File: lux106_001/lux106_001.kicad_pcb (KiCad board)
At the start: 2 copper layers, 19 parts, among them U1 40106, U2 LM324

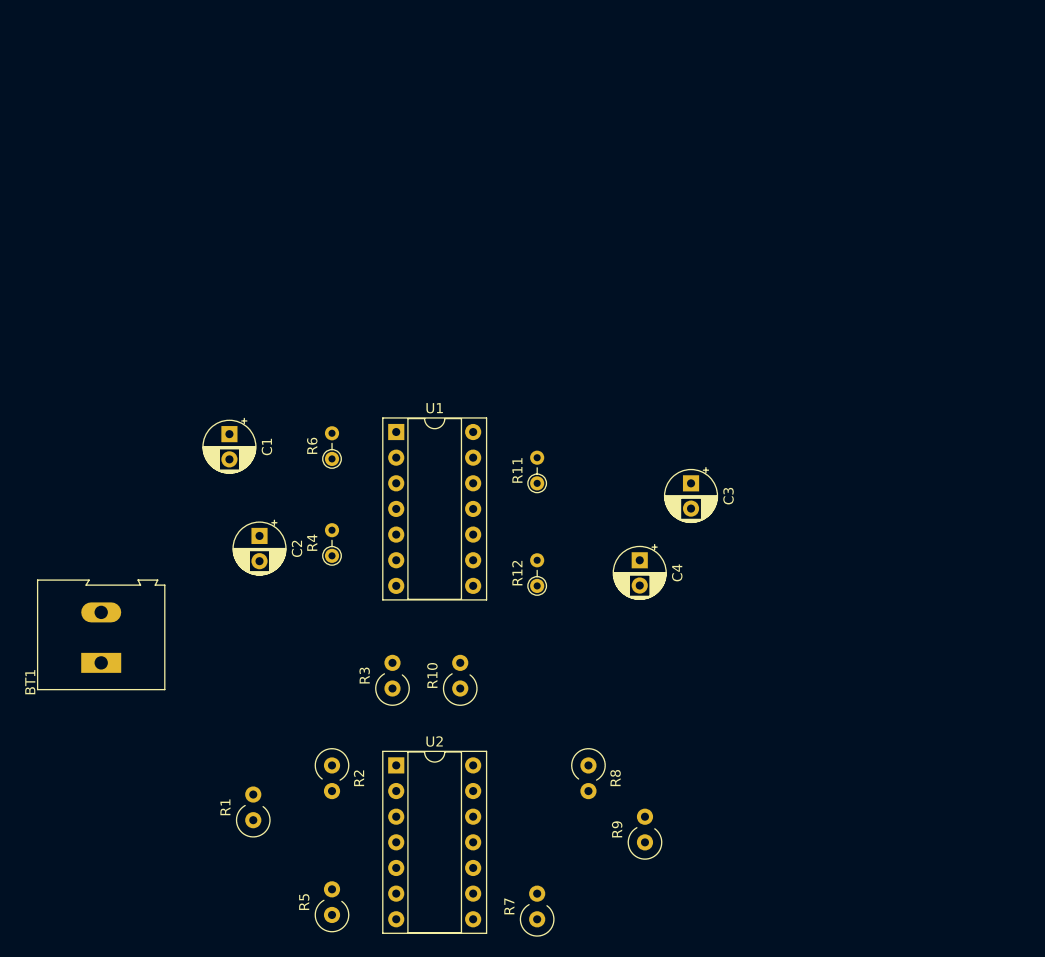
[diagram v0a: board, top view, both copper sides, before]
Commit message: update
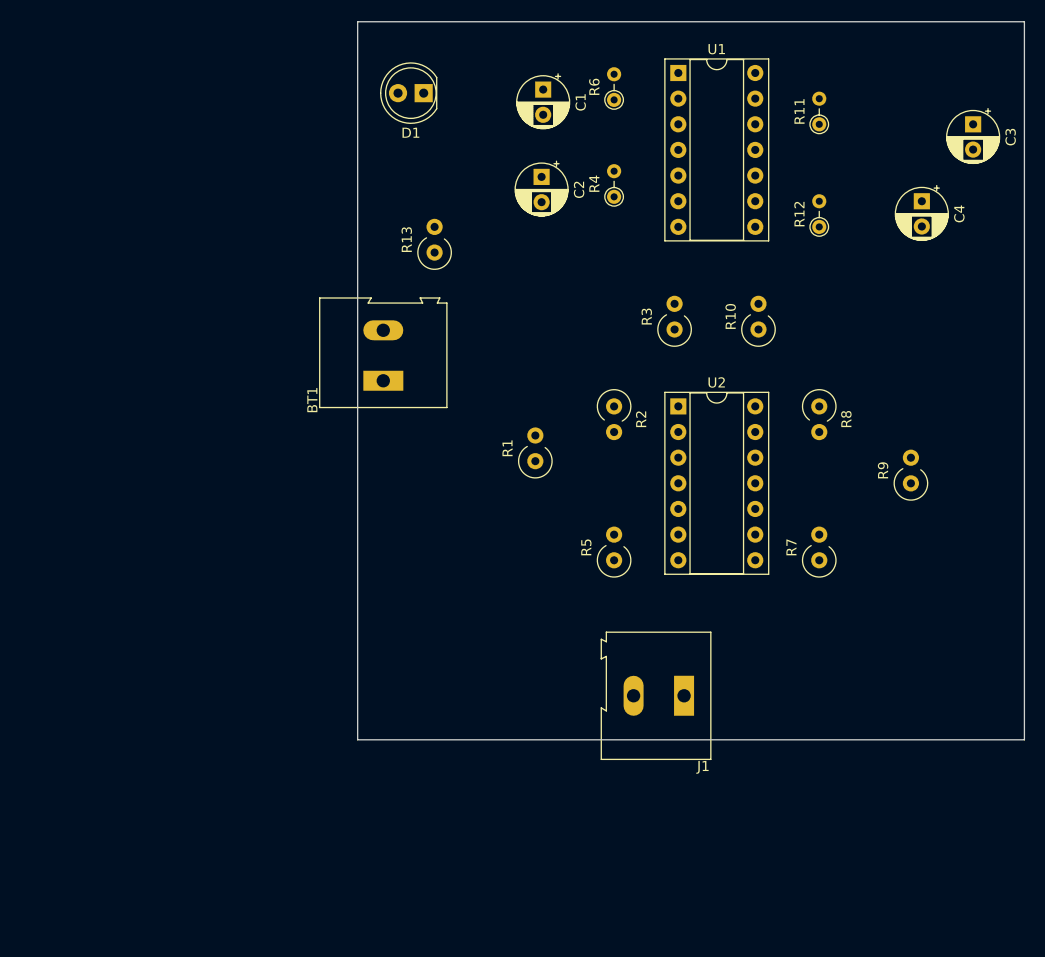
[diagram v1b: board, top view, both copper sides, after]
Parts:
- added D1: LED, LED_THT:LED_D5.0mm_Clear, F.Cu at (128.5, 63.0)
- added J1: Screw_Terminal_01x02, TerminalBlock:TerminalBlock_Altech_AK300-2_P5.00mm, F.Cu at (154.2, 122.6)
- added R13: 1k, Resistor_THT:R_Axial_DIN0309_L9.0mm_D3.2mm_P2.54mm_Vertical, F.Cu at (129.5, 78.7)
- moved R10 46.2 mm to (161.6, 86.4)
- moved C1 46.2 mm to (140.3, 62.6)
- moved R6 45.2 mm to (147.3, 63.6)
- moved U1 45.2 mm to (153.7, 61.0)
- moved U2 45.2 mm to (153.7, 94.0)
- moved C4 45.2 mm to (177.8, 73.7)
- moved R12 45.2 mm to (167.6, 76.2)
- moved R3 45.2 mm to (153.3, 86.4)
- moved R4 45.2 mm to (147.3, 73.2)
- moved R7 45.2 mm to (167.6, 109.2)
- moved C2 45.2 mm to (140.1, 71.2)
- moved C3 45.2 mm to (182.9, 66.0)
- moved R1 45.2 mm to (139.5, 99.4)
- moved R11 45.2 mm to (167.6, 66.0)
- moved R2 45.2 mm to (147.3, 94.0)
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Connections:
- R2 pad 1: Net-(R2-Pad1) -> OUT
- R5 pad 1: Net-(R5-Pad1) -> OUT
- R7 pad 1: Net-(R7-Pad1) -> OUT
- R8 pad 1: Net-(R8-Pad1) -> OUT
- U1 pad 14: unconnected-(U1-Pad14) -> VCC
- U1 pad 7: unconnected-(U1-Pad7) -> Earth
- U2 pad 1: Net-(R2-Pad1) -> OUT
- U2 pad 14: Net-(R8-Pad1) -> OUT
- U2 pad 7: Net-(R5-Pad1) -> OUT
- U2 pad 8: Net-(R7-Pad1) -> OUT
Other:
- board outline added: 66 x 71.1 mm

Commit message: update
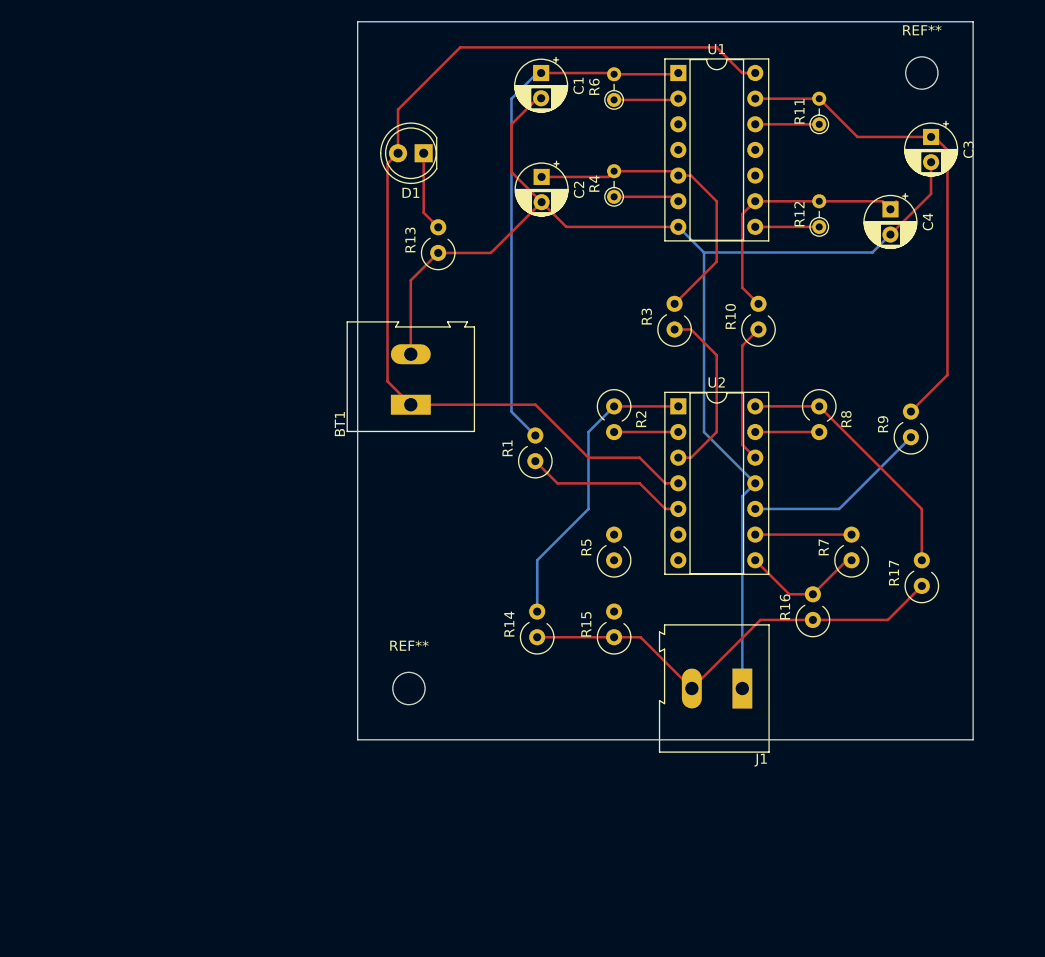
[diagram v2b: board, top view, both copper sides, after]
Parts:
- added R14: 1k, Resistor_THT:R_Axial_DIN0309_L9.0mm_D3.2mm_P2.54mm_Vertical, F.Cu at (139.7, 116.8)
- added R15: 1k, Resistor_THT:R_Axial_DIN0309_L9.0mm_D3.2mm_P2.54mm_Vertical, F.Cu at (147.3, 116.8)
- added R16: 1k, Resistor_THT:R_Axial_DIN0309_L9.0mm_D3.2mm_P2.54mm_Vertical, F.Cu at (167.0, 115.1)
- added R17: 1k, Resistor_THT:R_Axial_DIN0309_L9.0mm_D3.2mm_P2.54mm_Vertical, F.Cu at (177.8, 111.8)
- added REF**: MountingHole_3.2mm_M3, MountingHole:MountingHole_3.2mm_M3, F.Cu at (177.8, 61.0)
- added REF**: MountingHole_3.2mm_M3, MountingHole:MountingHole_3.2mm_M3, F.Cu at (127.0, 121.9)
- moved D1 5.95 mm to (128.5, 68.9)
- moved J1 5.81 mm to (160.0, 121.9)
- moved R9 4.57 mm to (176.7, 97.0)
- moved C3 4.35 mm to (178.7, 67.3)
- moved BT1 3.61 mm to (127.2, 93.8)
- moved C4 3.21 mm to (174.7, 74.5)
- moved R7 3.20 mm to (170.8, 109.2)
- moved C1 1.65 mm to (140.1, 61.0)
- moved R13 0.36 mm to (129.9, 78.8)
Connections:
- R2 pad 1: OUT -> Net-(R2-Pad1)
- R5 pad 1: OUT -> Net-(R5-Pad1)
- R7 pad 1: OUT -> Net-(R7-Pad1)
- R8 pad 1: OUT -> Net-(R8-Pad1)
- U2 pad 1: OUT -> Net-(R2-Pad1)
- U2 pad 14: OUT -> Net-(R8-Pad1)
- U2 pad 7: OUT -> Net-(R5-Pad1)
- U2 pad 8: OUT -> Net-(R7-Pad1)
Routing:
- net Earth: track 0.00 -> 128.0 mm
- net VCC: track 0.00 -> 99.3 mm
- net Net-(C1-Pad1): track 0.00 -> 52.0 mm
- net Net-(C3-Pad1): track 0.00 -> 48.6 mm
- net OUT: track 0.00 -> 44.4 mm
- net Net-(C2-Pad1): track 0.00 -> 30.7 mm
- net Net-(R2-Pad1): track 0.00 -> 29.8 mm
- net Net-(C4-Pad1): track 0.00 -> 26.1 mm
- net Net-(R8-Pad1): track 0.00 -> 25.8 mm
- net Net-(R9-Pad1): track 0.00 -> 18.4 mm
- net Net-(R3-Pad1): track 0.00 -> 17.7 mm
- net Net-(R1-Pad1): track 0.00 -> 16.1 mm
- net Net-(R10-Pad1): track 0.00 -> 13.9 mm
- net Net-(R7-Pad1): track 0.00 -> 12.3 mm
- net Net-(R7-Pad2): track 0.00 -> 9.54 mm
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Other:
- board size 66 x 71.1 mm -> 61 x 71.1 mm
